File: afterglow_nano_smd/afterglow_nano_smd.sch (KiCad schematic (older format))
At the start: 116 parts, among them J1 J137_IN_C, J2 J133_IN_R, J3 Conn_Power, J4 J133_OUT_R, J5 J137_OUT_C, J6 J134_OUT_R, J7 J138_OUT_C, J8 J135_OUT_R, J9 136_OUT_C, Q1 IRF5305, Q10 IRL2905, Q11 IRL2905, Q12 IRL2905, Q13 IRL2905, Q14 IRL2905, Q15 IRL2905, Q16 IRL2905, Q2 IRF5305, Q3 IRF5305, Q4 IRF5305, Q5 IRF5305, Q6 IRF5305, Q7 IRF5305, Q8 IRF5305, Q9 IRL2905, SW1 CFG, U1 74LS165, U2 74LS165, U3 5V_Regulator, U5 74HC595, U6 74HC595, U7 ULN2803A

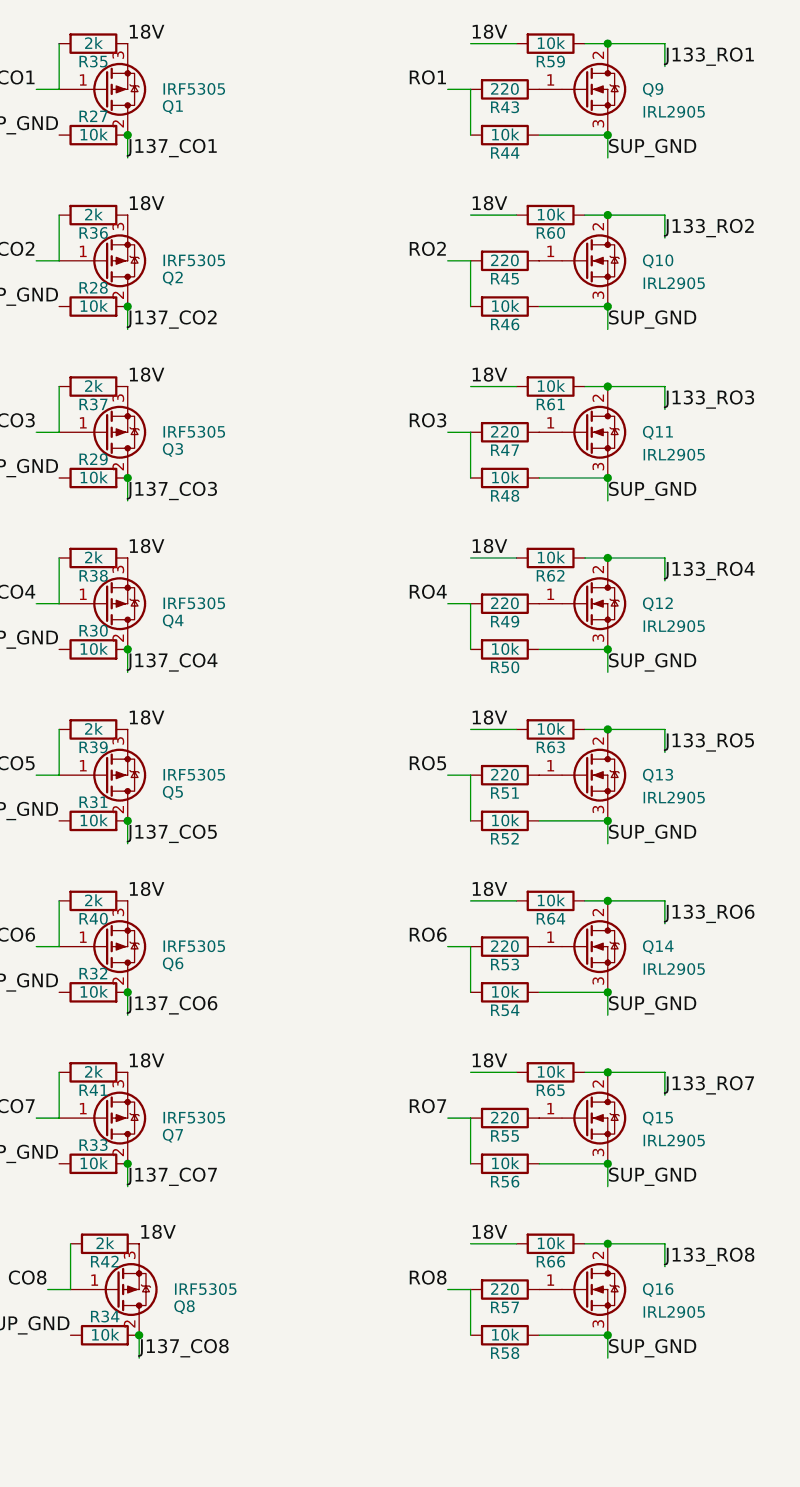
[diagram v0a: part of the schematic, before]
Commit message: Minor schematic updates
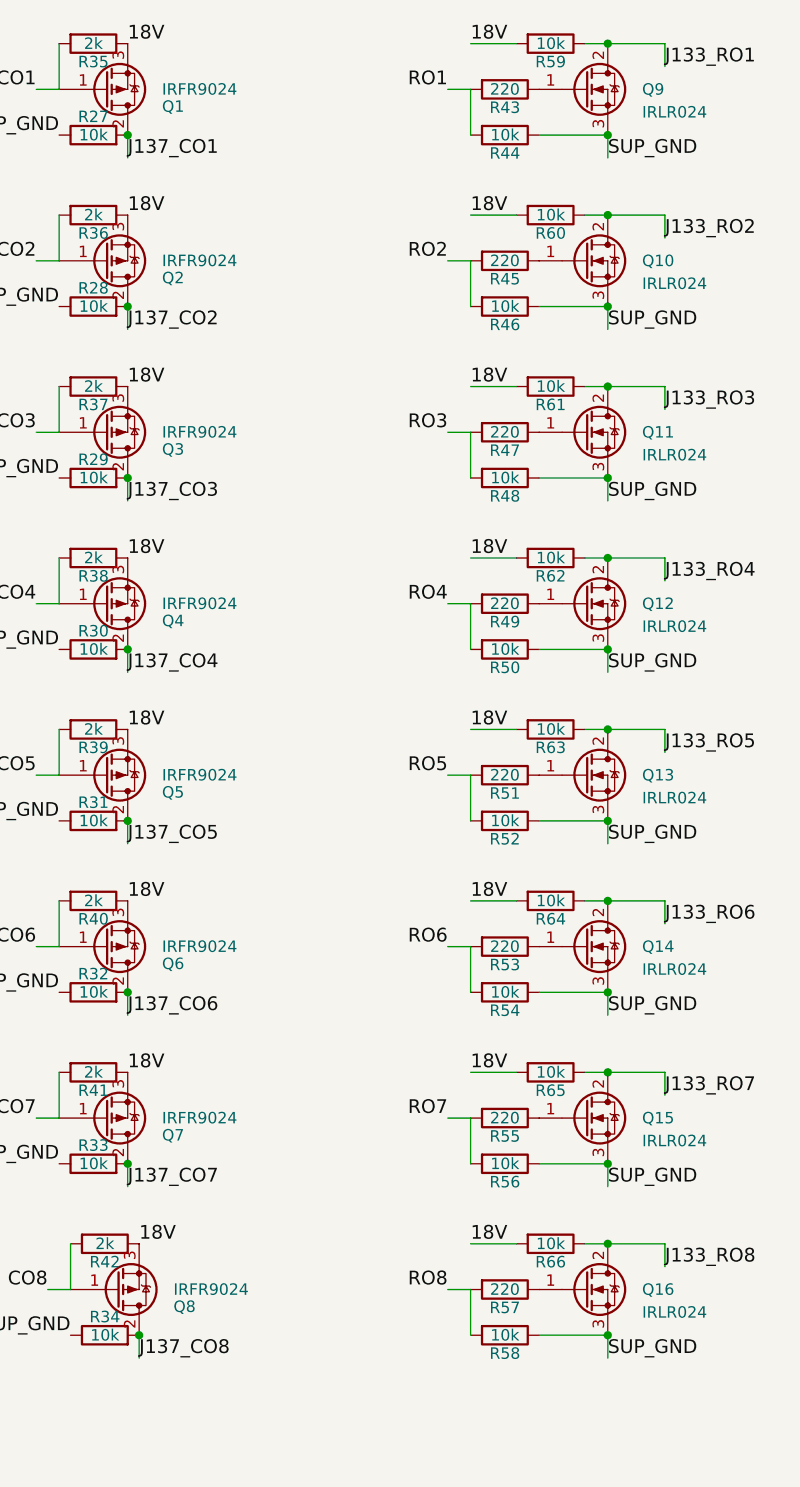
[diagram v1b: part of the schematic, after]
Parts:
- Q1, Q2, Q3, Q4, Q5, Q6, Q7, Q8: value IRF5305 -> IRFR9024
- Q10, Q11, Q12, Q13, Q14, Q15, Q16, Q9: value IRL2905 -> IRLR024
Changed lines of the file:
@@
 P 8100 850
 F 0 "Q1" H 8350 925 50  0000 L CNN
-F 1 "IRF5305" H 8350 850 50  0000 L CNN
+F 1 "IRFR9024" H 8350 850 50  0000 L CNN
 F 2 "TO_SOT_Packages_SMD:TO-252-2" H 8350 775 50  0001 L CIN
 F 3 "" H 8100 850 50  0001 L CNN
@@
 P 8100 1600
 F 0 "Q2" H 8350 1675 50  0000 L CNN
-F 1 "IRF5305" H 8350 1600 50  0000 L CNN
+F 1 "IRFR9024" H 8350 1600 50  0000 L CNN
 F 2 "TO_SOT_Packages_SMD:TO-252-2" H 8350 1525 50  0001 L CIN
 F 3 "" H 8100 1600 50  0001 L CNN
@@
 P 8100 2350
 F 0 "Q3" H 8350 2425 50  0000 L CNN
-F 1 "IRF5305" H 8350 2350 50  0000 L CNN
+F 1 "IRFR9024" H 8350 2350 50  0000 L CNN
 F 2 "TO_SOT_Packages_SMD:TO-252-2" H 8350 2275 50  0001 L CIN
 F 3 "" H 8100 2350 50  0001 L CNN
@@
 P 8100 3100
 F 0 "Q4" H 8350 3175 50  0000 L CNN
-F 1 "IRF5305" H 8350 3100 50  0000 L CNN
+F 1 "IRFR9024" H 8350 3100 50  0000 L CNN
 F 2 "TO_SOT_Packages_SMD:TO-252-2" H 8350 3025 50  0001 L CIN
 F 3 "" H 8100 3100 50  0001 L CNN
@@
 P 8100 3850
 F 0 "Q5" H 8350 3925 50  0000 L CNN
-F 1 "IRF5305" H 8350 3850 50  0000 L CNN
+F 1 "IRFR9024" H 8350 3850 50  0000 L CNN
 F 2 "TO_SOT_Packages_SMD:TO-252-2" H 8350 3775 50  0001 L CIN
 F 3 "" H 8100 3850 50  0001 L CNN
@@
 P 8100 4600
 F 0 "Q6" H 8350 4675 50  0000 L CNN
-F 1 "IRF5305" H 8350 4600 50  0000 L CNN
+F 1 "IRFR9024" H 8350 4600 50  0000 L CNN
 F 2 "TO_SOT_Packages_SMD:TO-252-2" H 8350 4525 50  0001 L CIN
 F 3 "" H 8100 4600 50  0001 L CNN
@@
 P 8100 5350
 F 0 "Q7" H 8350 5425 50  0000 L CNN
-F 1 "IRF5305" H 8350 5350 50  0000 L CNN
+F 1 "IRFR9024" H 8350 5350 50  0000 L CNN
 F 2 "TO_SOT_Packages_SMD:TO-252-2" H 8350 5275 50  0001 L CIN
 F 3 "" H 8100 5350 50  0001 L CNN
@@
 P 8150 6100
 F 0 "Q8" H 8400 6175 50  0000 L CNN
-F 1 "IRF5305" H 8400 6100 50  0000 L CNN
+F 1 "IRFR9024" H 8400 6100 50  0000 L CNN
 F 2 "TO_SOT_Packages_SMD:TO-252-2" H 8400 6025 50  0001 L CIN
 F 3 "" H 8150 6100 50  0001 L CNN
@@
 P 10200 850
 F 0 "Q9" H 10450 850 50  0000 L CNN
-F 1 "IRL2905" H 10450 750 50  0000 L CNN
+F 1 "IRLR024" H 10450 750 50  0000 L CNN
 F 2 "TO_SOT_Packages_SMD:TO-252-2" H 10450 775 50  0001 L CIN
 F 3 "" H 10200 850 50  0001 L CNN
@@
 P 10200 1600
 F 0 "Q10" H 10450 1600 50  0000 L CNN
-F 1 "IRL2905" H 10450 1500 50  0000 L CNN
+F 1 "IRLR024" H 10450 1500 50  0000 L CNN
 F 2 "TO_SOT_Packages_SMD:TO-252-2" H 10450 1525 50  0001 L CIN
 F 3 "" H 10200 1600 50  0001 L CNN
@@
 P 10200 2350
 F 0 "Q11" H 10450 2350 50  0000 L CNN
-F 1 "IRL2905" H 10450 2250 50  0000 L CNN
+F 1 "IRLR024" H 10450 2250 50  0000 L CNN
 F 2 "TO_SOT_Packages_SMD:TO-252-2" H 10450 2275 50  0001 L CIN
 F 3 "" H 10200 2350 50  0001 L CNN
@@
 P 10200 3100
 F 0 "Q12" H 10450 3100 50  0000 L CNN
-F 1 "IRL2905" H 10450 3000 50  0000 L CNN
+F 1 "IRLR024" H 10450 3000 50  0000 L CNN
 F 2 "TO_SOT_Packages_SMD:TO-252-2" H 10450 3025 50  0001 L CIN
 F 3 "" H 10200 3100 50  0001 L CNN
@@
 P 10200 3850
 F 0 "Q13" H 10450 3850 50  0000 L CNN
-F 1 "IRL2905" H 10450 3750 50  0000 L CNN
+F 1 "IRLR024" H 10450 3750 50  0000 L CNN
 F 2 "TO_SOT_Packages_SMD:TO-252-2" H 10450 3775 50  0001 L CIN
 F 3 "" H 10200 3850 50  0001 L CNN
@@
 P 10200 4600
 F 0 "Q14" H 10450 4600 50  0000 L CNN
-F 1 "IRL2905" H 10450 4500 50  0000 L CNN
+F 1 "IRLR024" H 10450 4500 50  0000 L CNN
 F 2 "TO_SOT_Packages_SMD:TO-252-2" H 10450 4525 50  0001 L CIN
 F 3 "" H 10200 4600 50  0001 L CNN
@@
 P 10200 5350
 F 0 "Q15" H 10450 5350 50  0000 L CNN
-F 1 "IRL2905" H 10450 5250 50  0000 L CNN
+F 1 "IRLR024" H 10450 5250 50  0000 L CNN
 F 2 "TO_SOT_Packages_SMD:TO-252-2" H 10450 5275 50  0001 L CIN
 F 3 "" H 10200 5350 50  0001 L CNN
@@
 P 10200 6100
 F 0 "Q16" H 10450 6100 50  0000 L CNN
-F 1 "IRL2905" H 10450 6000 50  0000 L CNN
+F 1 "IRLR024" H 10450 6000 50  0000 L CNN
 F 2 "TO_SOT_Packages_SMD:TO-252-2" H 10450 6025 50  0001 L CIN
 F 3 "" H 10200 6100 50  0001 L CNN
